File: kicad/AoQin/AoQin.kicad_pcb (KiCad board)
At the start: 2 copper layers, 111.2 x 81 mm, 11 parts, among them J1 Conn_02x03_Odd_Even, J2 Conn_02x03_Odd_Even, J3 Screw_Terminal_01x12, J7 Screw_Terminal_01x12, J8 Screw_Terminal_01x03, J9 Screw_Terminal_01x03

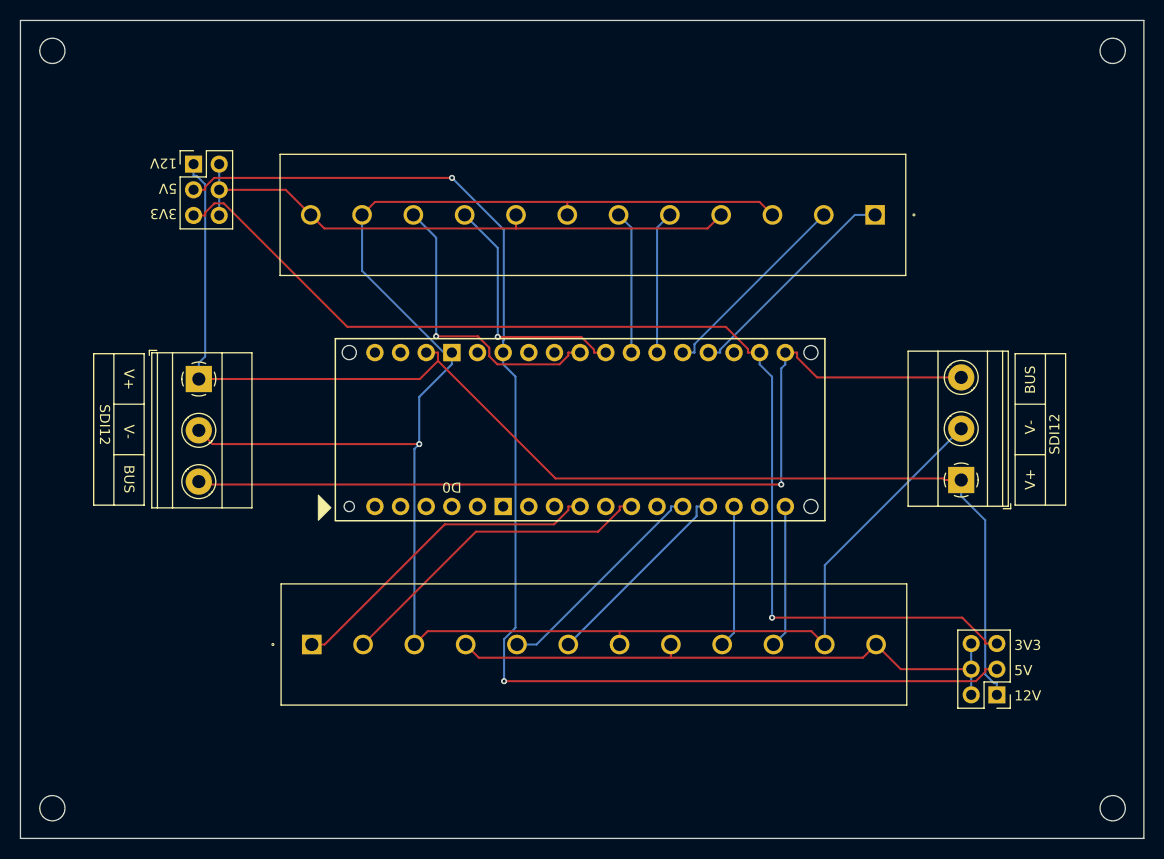
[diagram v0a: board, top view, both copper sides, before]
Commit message: Web of Desire
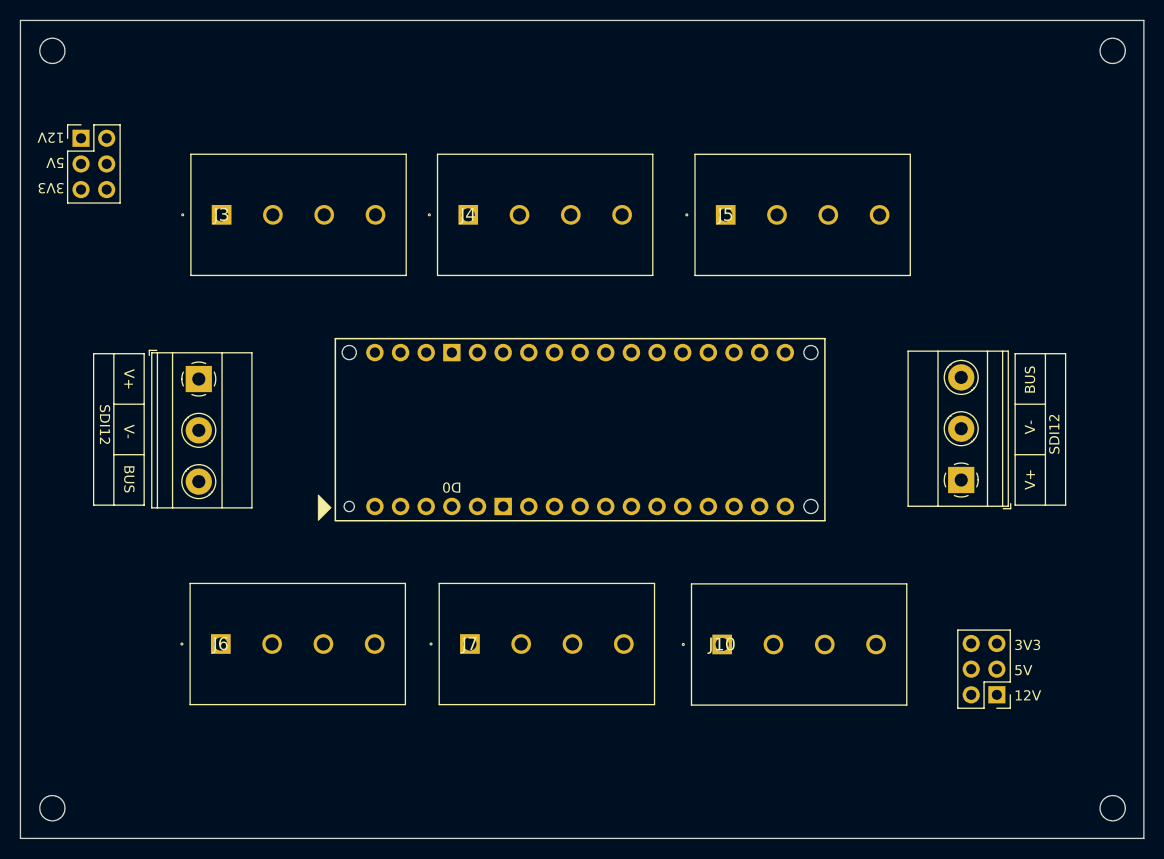
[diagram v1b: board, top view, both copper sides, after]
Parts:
- added J10: 1869237, footprints:SMKDSN_15_4_508, F.Cu at (101.8, 79.3)
- added J4: 1869237, footprints:SMKDSN_15_4_508, F.Cu at (76.7, 36.7)
- added J5: 1869237, footprints:SMKDSN_15_4_508, F.Cu at (102.2, 36.7)
- added J6: 1869237, footprints:SMKDSN_15_4_508, F.Cu at (52.2, 79.2)
- J3, J7: value Screw_Terminal_01x12 -> 1869237; footprint footprints:1869318 -> footprints:SMKDSN_15_4_508
- moved J7 58.4 mm to (76.8, 79.2), turned to 0 degrees
- moved J3 43.5 mm to (52.3, 36.7)
- moved J1 11.4 mm to (38.3, 29.2)
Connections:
- J3 pad 1: /A6 -> /A0
- J3 pad 2: /A7 -> /A6
- J3 pad 4: /VIN2 -> /VIN1
- J7 pad 1: /A0 -> /A4
- J7 pad 2: /A1 -> /A10
- J7 pad 4: /VIN1 -> /VIN2
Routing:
- net GND: track 183.8 -> 0.00 mm, vias 1 -> 0
- net /5V: track 128.7 -> 0.00 mm, vias 2 -> 0
- net +12V: track 128.2 -> 0.00 mm
- net /3V3: track 113.3 -> 0.00 mm, vias 1 -> 0
- net /D13: track 89.8 -> 0.00 mm, vias 1 -> 0
- net /VIN2: track 58.5 -> 0.00 mm
- net /VIN1: track 58.3 -> 0.00 mm
- net /A7: track 32.4 -> 0.00 mm
- net /A6: track 32.4 -> 0.00 mm
- net /A5: track 29.5 -> 0.00 mm, vias 1 -> 0
- net /A4: track 25.0 -> 0.00 mm, vias 1 -> 0
- net /A0: track 22.3 -> 0.00 mm
- net /A8: track 22.3 -> 0.00 mm
- net /A1: track 20.1 -> 0.00 mm
- net /A9: track 20.1 -> 0.00 mm
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
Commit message: Two Men and a Baby
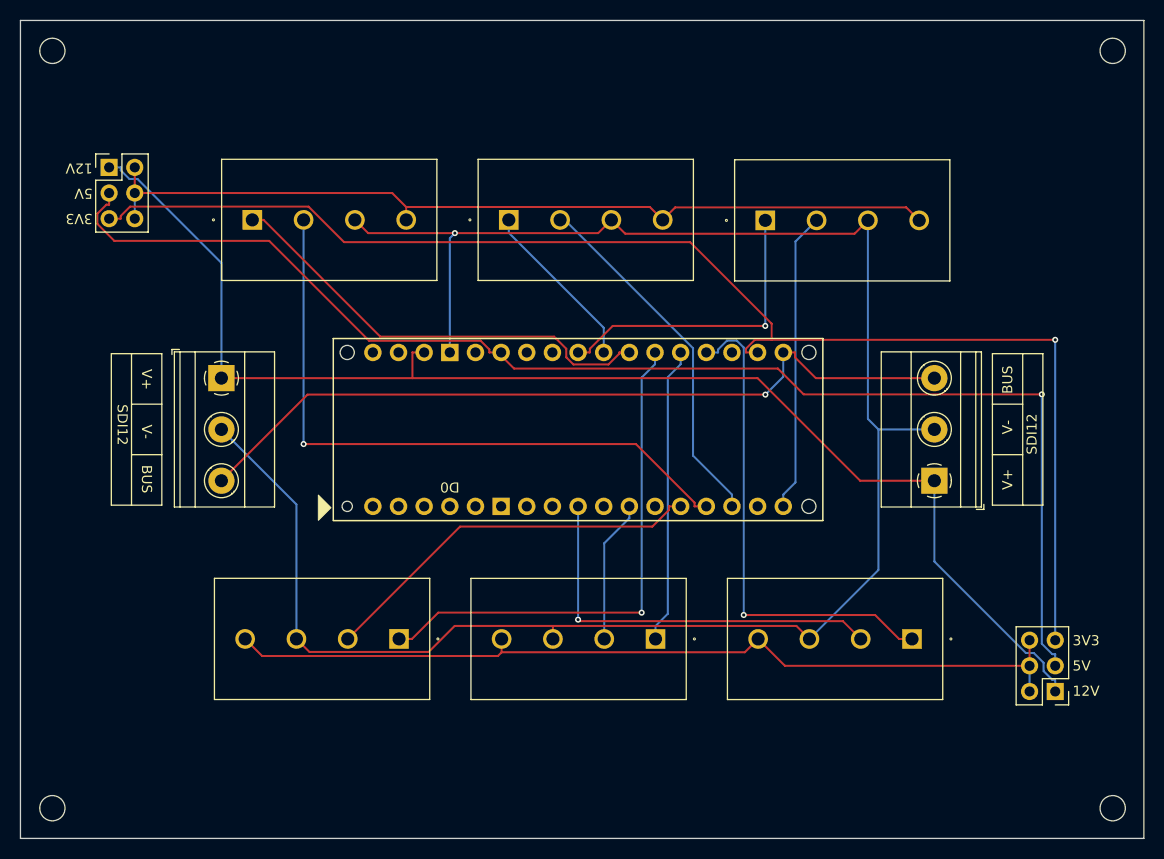
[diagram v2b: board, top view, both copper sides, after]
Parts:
- moved J1 110.9 mm to (134.8, 83.9), turned to 180 degrees
- moved J2 102.3 mm to (41.1, 32.0), turned to 0 degrees
- moved J3 80.2 mm to (120.6, 78.7), turned to 180 degrees
- moved J5 53.0 mm to (69.8, 78.7), turned to 180 degrees
- moved J4 45.9 mm to (95.2, 78.7), turned to 180 degrees
- moved J10 42.2 mm to (106.1, 37.3)
- moved J7 42.2 mm to (80.7, 37.2)
- moved J6 42.1 mm to (55.3, 37.2)
- moved J9 2.66 mm to (122.8, 63.1)
- moved J8 2.24 mm to (52.2, 52.9)
- moved A1 0.20 mm to (111.8, 49.0)
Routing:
- net GND: track 0.00 -> 193.3 mm, vias 0 -> 1
- net /3V3: track 0.00 -> 134.9 mm, vias 0 -> 1
- net /5V: track 0.00 -> 132.3 mm, vias 0 -> 1
- net +12V: track 0.00 -> 131.6 mm
- net /VIN1: track 0.00 -> 86.6 mm
- net /VIN2: track 0.00 -> 86.2 mm
- net /D13: track 0.00 -> 78.6 mm, vias 0 -> 1
- net /A9: track 0.00 -> 64.8 mm, vias 0 -> 1
- net /A2: track 0.00 -> 51.4 mm, vias 0 -> 1
- net /A0: track 0.00 -> 48.8 mm, vias 0 -> 1
- net /A3: track 0.00 -> 44.3 mm
- net /A6: track 0.00 -> 40.0 mm, vias 0 -> 1
- net /A8: track 0.00 -> 38.6 mm
- net /A10: track 0.00 -> 35.7 mm
- net /A5: track 0.00 -> 30.3 mm, vias 0 -> 1
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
